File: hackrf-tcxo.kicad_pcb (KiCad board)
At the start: 2 copper layers, 20 x 20 mm, 2 parts, among them J1 Conn_02x07_Odd_Even, U1 TXC_7N(10)

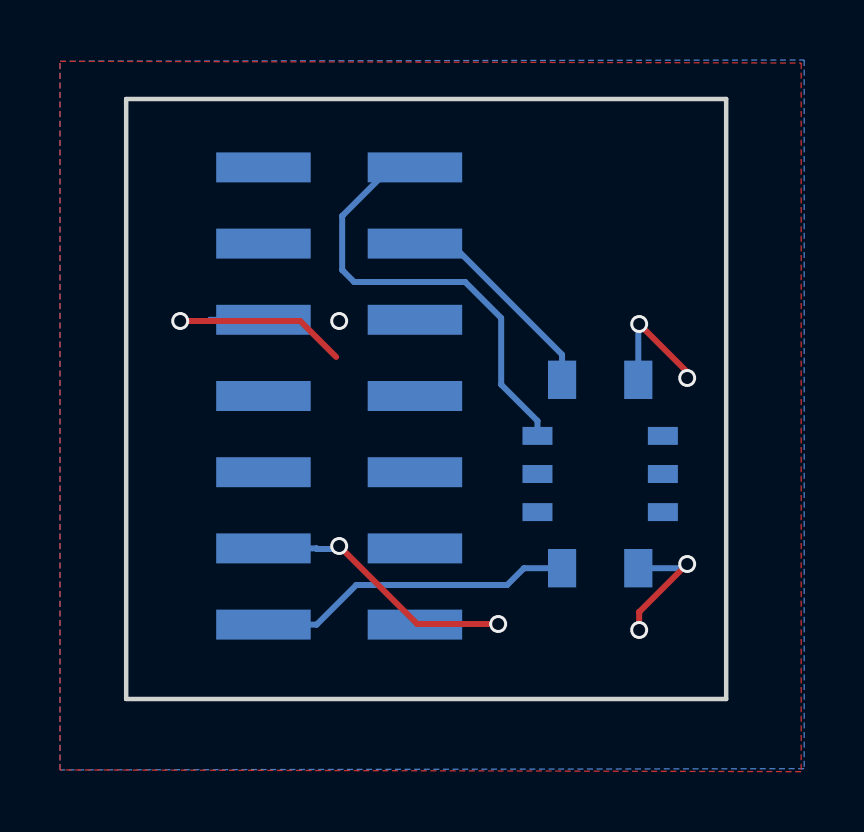
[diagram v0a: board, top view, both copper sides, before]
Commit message: v1
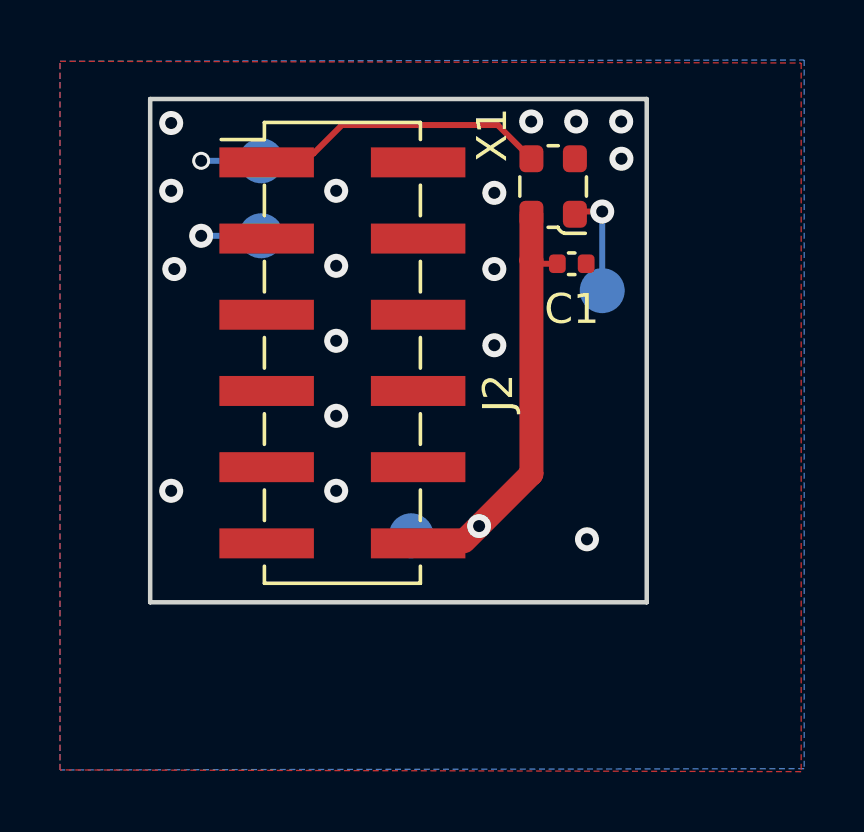
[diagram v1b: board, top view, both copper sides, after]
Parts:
- removed J1: Conn_02x07_Odd_Even, Pin_Headers:Pin_Header_Straight_2x07_Pitch2.54mm_SMD
- removed U1: TXC_7N(10), hackrf-tcxo:TXC_7N(10)
- added C1: 100n, Capacitor_SMD:C_0402_1005Metric, F.Cu at (146.9, 101.5)
- added J2: Conn_02x06_Odd_Even, Connector_PinHeader_2.54mm:PinHeader_2x06_P2.54mm_Vertical_SMD, F.Cu at (139.2, 104.5)
- added TP1: EN, TestPoint:TestPoint_Pad_D1.5mm, B.Cu at (147.9, 102.4)
- added TP2: CLK, TestPoint:TestPoint_Pad_D1.5mm, B.Cu at (136.5, 98.1)
- added TP3: GND, TestPoint:TestPoint_Pad_D1.5mm, B.Cu at (136.5, 100.6)
- added TP4: VCC, TestPoint:TestPoint_Pad_D1.5mm, B.Cu at (141.5, 110.6)
- added X1: ECS-2520MV-100-AN-TR, Oscillator:Oscillator_SMD_ECS_2520MV-xxx-xx-4Pin_2.5x2.0mm, F.Cu at (146.2, 98.9)
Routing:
- net GND: track 26.3 -> 2.00 mm, vias 8 -> 18
- net EN: track 15.3 -> 3.59 mm, vias 0 -> 1
- net VCC: track 7.28 -> 15.1 mm, vias 0 -> 1
- net HRF_CLKIN: track 10.7 -> 11.9 mm, vias 0 -> 1
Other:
- board size 20 x 20 mm -> 16.6 x 16.8 mm
- net class Default removed
